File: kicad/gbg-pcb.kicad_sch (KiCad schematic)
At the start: 49 parts, among them IC2 D78B05T-1.0, J1 9 2.54mm pitch header pins, J12 screw terminal, J2 Conn_01x02, J3 VP0265840000G, J4 Screw_Terminal_01x04, J5 Screw_Terminal_01x03, J8 1017514, J9 1017514, P1 rpi pico, Q1 PSMN1R2-25YLDX, Q2 PSMN1R2-25YLDX, Q3 PSMN1R2-25YLDX, Q4 PSMN1R2-25YLDX, SW1 screw terminal, U1 IFX007TAUMA1, U2 IFX007TAUMA1, U3 IFX007TAUMA1, U4 IFX007TAUMA1

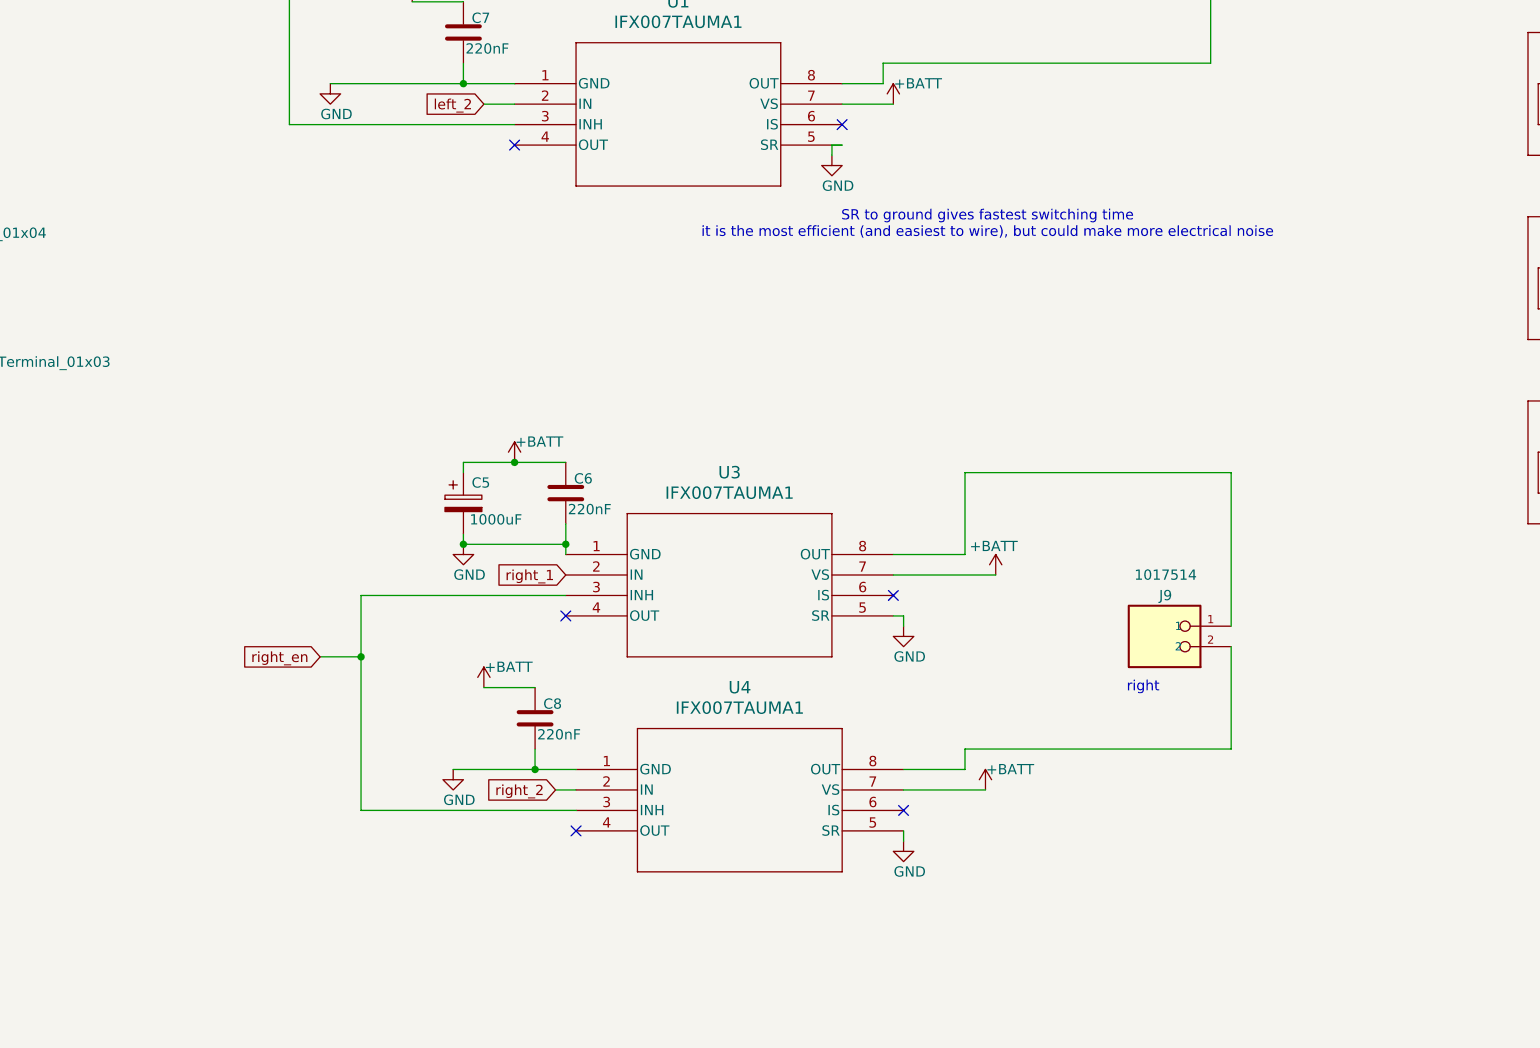
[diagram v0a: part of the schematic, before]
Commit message: adjust layout
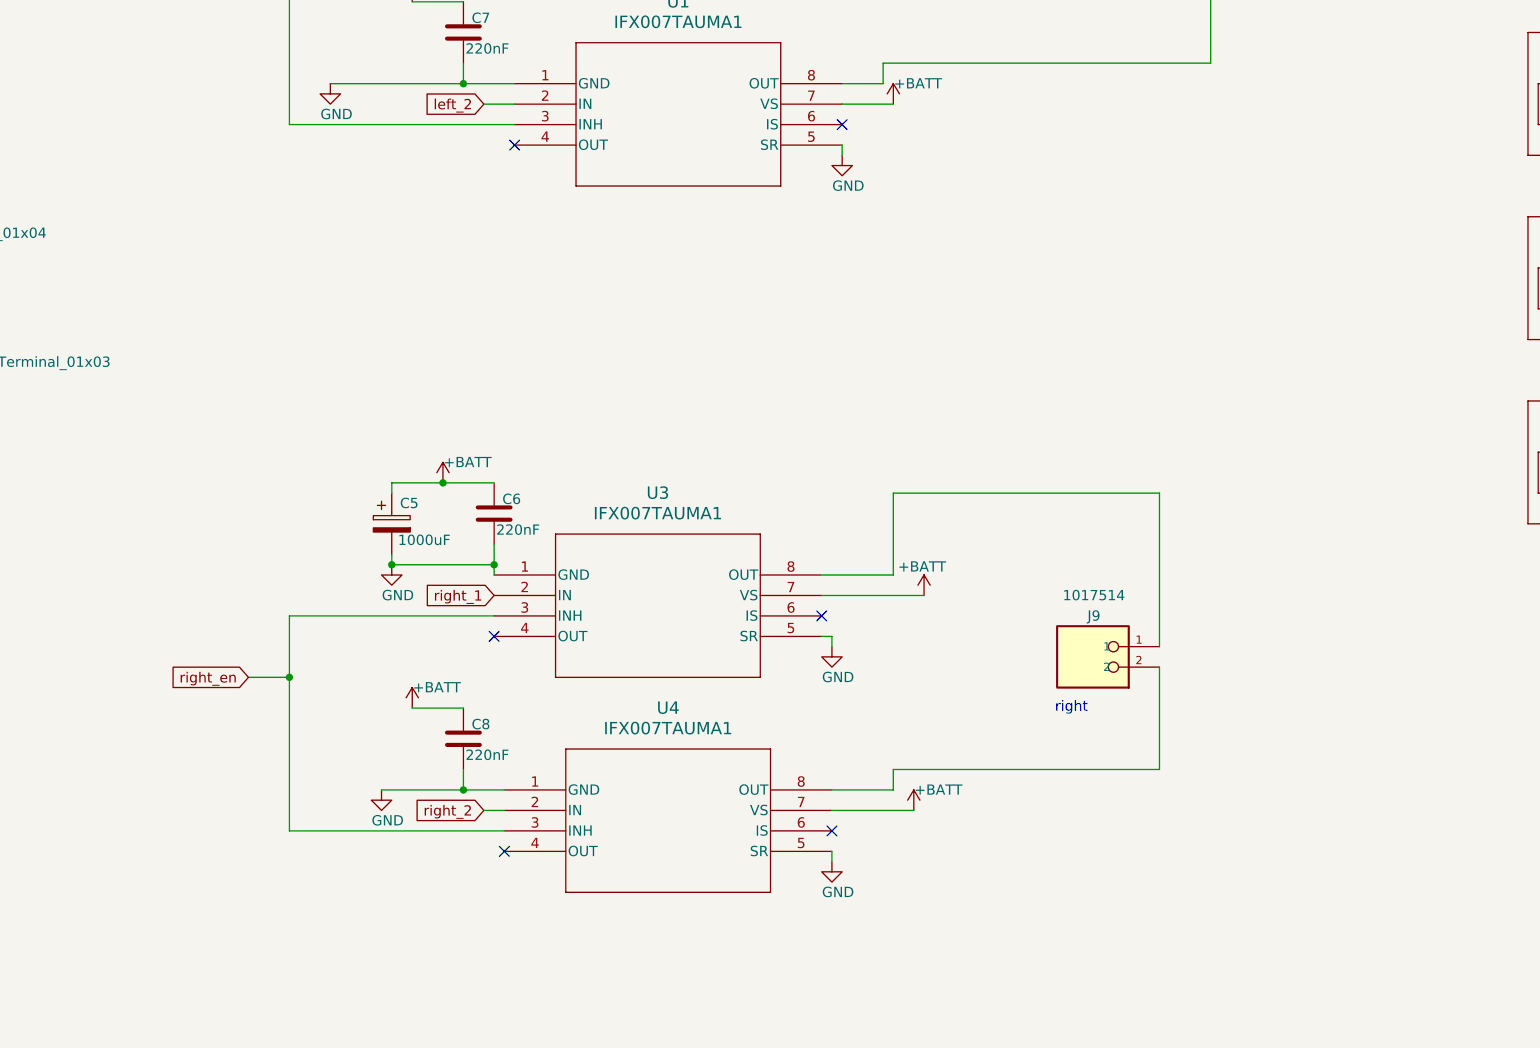
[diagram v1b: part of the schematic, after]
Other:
- note removed: "SR to ground gives fastest switching time it is the most efficient (and easiest to wire), but could make more electrical noise"
- moved on the sheet: C5, C6, C8, J9, U3, U4
